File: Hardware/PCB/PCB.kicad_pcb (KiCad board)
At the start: 4 copper layers, 130 x 65 mm, 106 parts, among them IC3 MPX5500DP, IC4 MPX5500DP, J1 DC Motor Terminal, J18 Programmer, J2 Solenoid Terminal, J3 Brushless Vac Motor, J4 54-00127, J5 Brushless Pump Motor, Q1 MMBT2222A, Q2 MMBT2222A, Q3 MMBT2222A, Q4 MMBT2222A, Q5 MMBT2222A, Q6 MMBT2222A, U1 ER-TFTM032-3, U10 AZ1117-5.0, U11 ESP32-S3-WROOM-1U-N16R8, U2 ADS1219IPWR, U3 DRV8871DDA, U4 AP7361C-33E, U5 74LVC2T45DC, U6 TPS7A2050PDBVR, U7 DS3232M, U8 DRV8871DDA

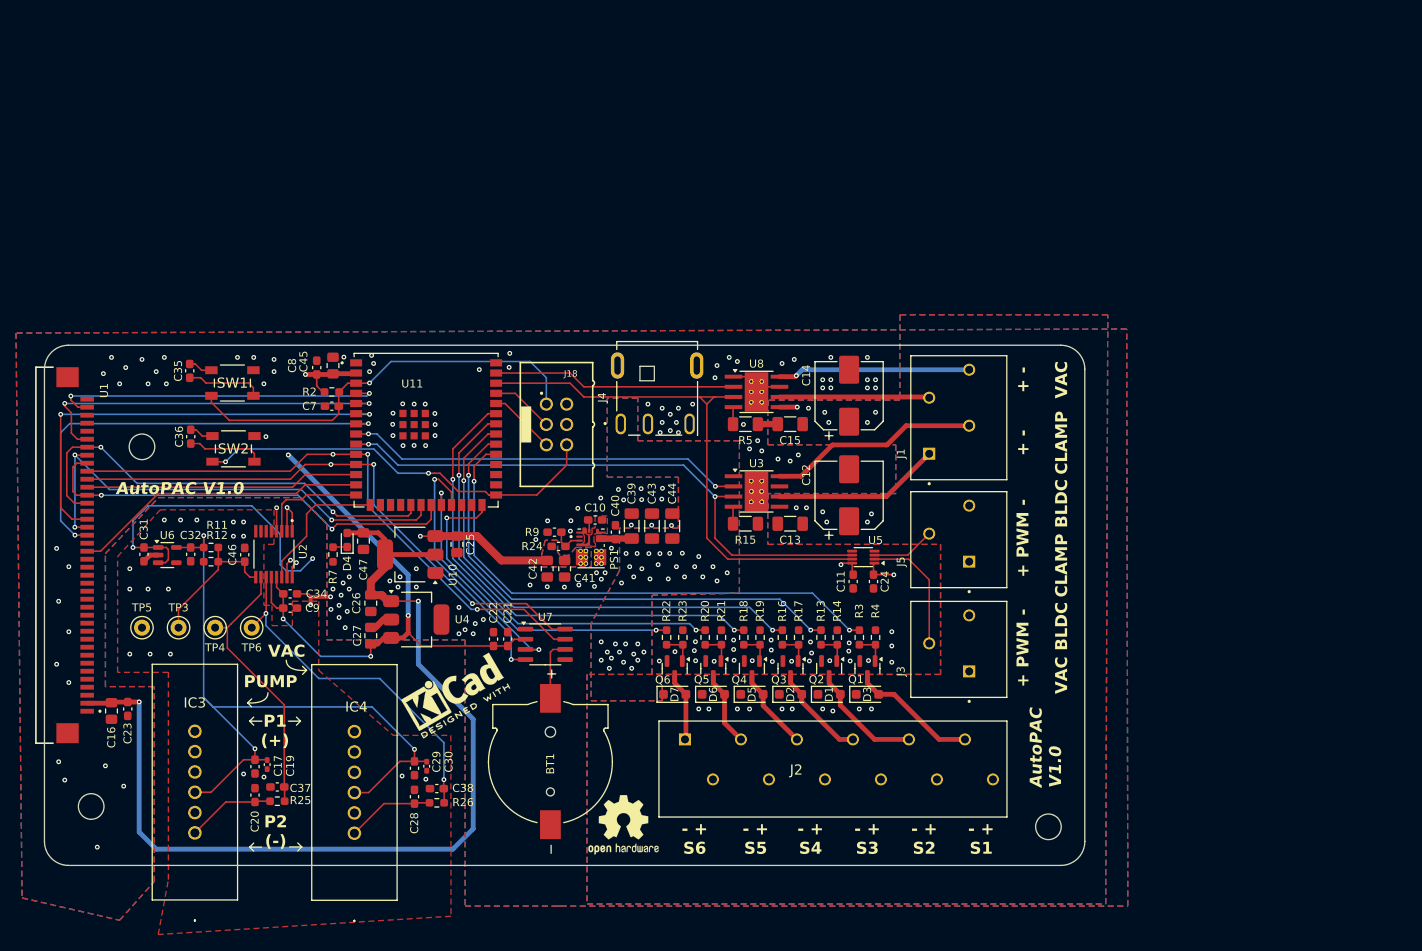
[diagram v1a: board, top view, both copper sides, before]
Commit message: done with this, placed order
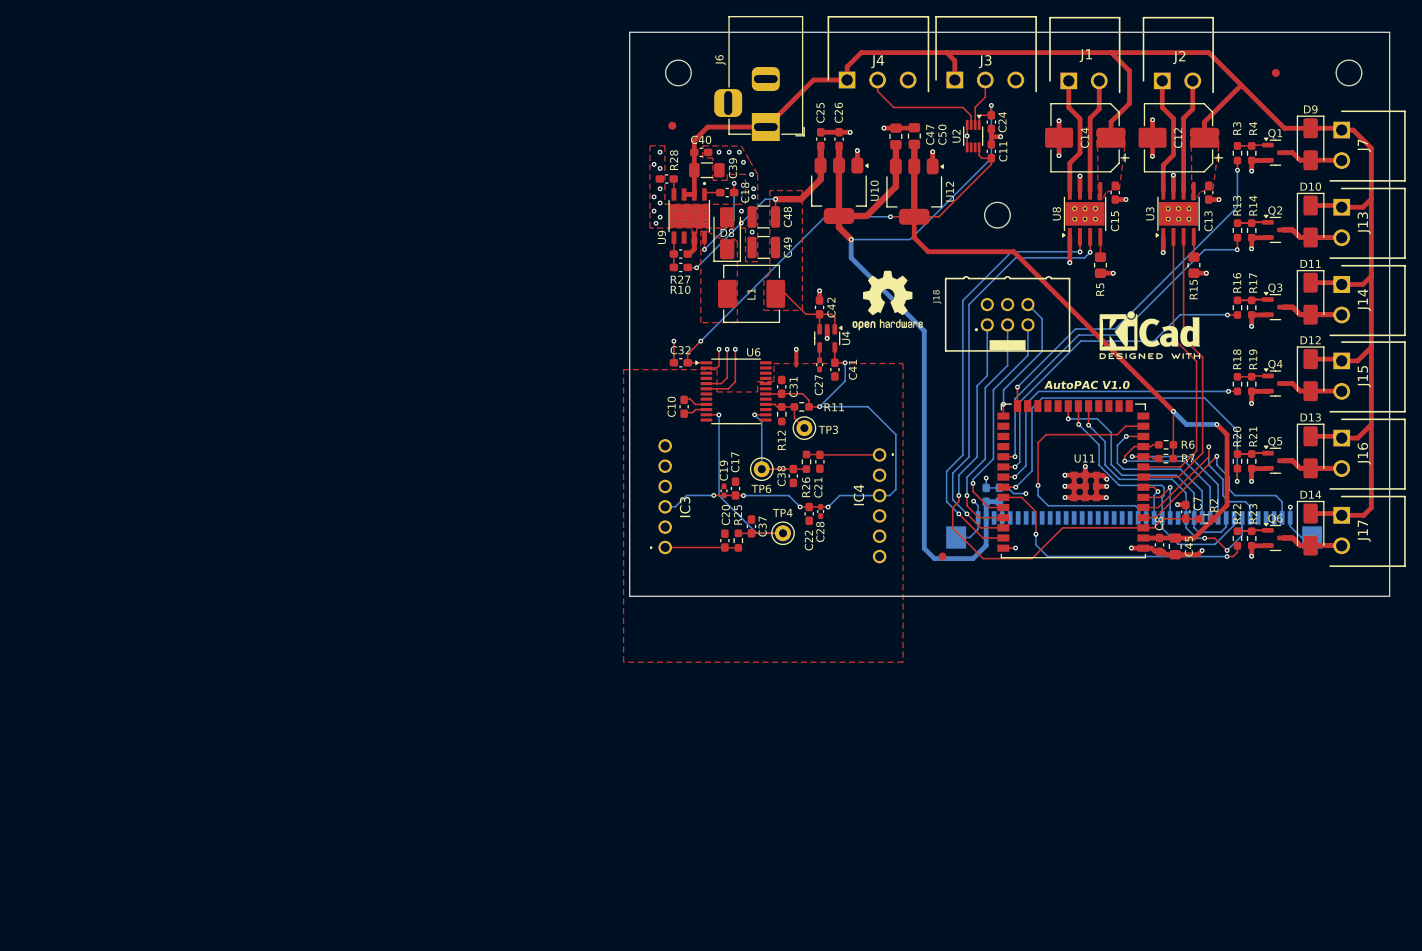
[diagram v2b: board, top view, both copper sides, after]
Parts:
- removed BT1: 1056, Vendor_Footprints:BAT_1056
- removed C29: 1uF, Capacitor_SMD:C_0603_1608Metric_Pad1.08x0.95mm_HandSolder
- removed C30: 0.01uF, Capacitor_SMD:C_0402_1005Metric_Pad0.74x0.62mm_HandSolder
- removed C34, C35, C36, C46, C9: 0.1u, Capacitor_SMD:C_0603_1608Metric_Pad1.08x0.95mm_HandSolder
- removed C43, C44: 10uF, Capacitor_SMD:C_1206_3216Metric_Pad1.33x1.80mm_HandSolder
- removed D1, D2, D3, D5, D6, D7: SMD110PL-TP, Diode_SMD:D_SOD-123F
- removed D4: LED, LED_SMD:LED_0603_1608Metric_Pad1.05x0.95mm_HandSolder
- removed H3: MountingHole, MountingHole:MountingHole_3.2mm_M3
- removed J5: Brushless Pump Motor, Vendor_Footprints:TE_1985205
- removed PS1: TPSM84338RCJR, Vendor_Footprints:CONV_TPSM84338RCJR
- removed R24: 82k, Capacitor_SMD:C_0603_1608Metric_Pad1.08x0.95mm_HandSolder
- removed R9: 10k, Capacitor_SMD:C_0603_1608Metric_Pad1.08x0.95mm_HandSolder
- removed SW1, SW2: ~, Vendor_Footprints:PTS647SN50SMTR2LFS
- removed TP5: TestPoint_Probe, TestPoint:TestPoint_Keystone_5000-5004_Miniature
- removed U5: 74LVC2T45DC, Package_SO:VSSOP-8_2.3x2mm_P0.5mm
- removed U7: DS3232M, Package_SO:SOIC-8_3.9x4.9mm_P1.27mm
- added C18: 100nF, Capacitor_SMD:C_0603_1608Metric_Pad1.08x0.95mm_HandSolder, F.Cu at (187.7, 49.8)
- added C48: 47uF, Capacitor_SMD:C_1210_3225Metric, F.Cu at (192.3, 52.8)
- added C49: 47uF, Capacitor_SMD:C_1210_3225Metric, F.Cu at (192.3, 56.6)
- added C50: 22uF, Capacitor_SMD:C_0805_2012Metric_Pad1.18x1.45mm_HandSolder, F.Cu at (211.1, 42.7)
- added D10: SS310, Diode_SMD:D_SMA, F.Cu at (260.6, 53.4)
- added D11: SS310, Diode_SMD:D_SMA, F.Cu at (260.6, 63.0)
- added D12: SS310, Diode_SMD:D_SMA, F.Cu at (260.6, 72.6)
- added D13: SS310, Diode_SMD:D_SMA, F.Cu at (260.6, 82.2)
- added D14: SS310, Diode_SMD:D_SMA, F.Cu at (260.6, 91.9)
- added D8: SS310, Diode_SMD:D_SMA, F.Cu at (187.7, 54.8)
- added D9: SS310, Diode_SMD:D_SMA, F.Cu at (260.6, 43.7)
- added H2: MountingHole, MountingHole:MountingHole_3.2mm_M3, F.Cu at (221.5, 52.6)
- added J13: Solenoid Terminal, Vendor_Footprints:CONN_WJ15EDGRC-3.81-2P, F.Cu at (264.5, 51.6)
- added J14: Solenoid Terminal, Vendor_Footprints:CONN_WJ15EDGRC-3.81-2P, F.Cu at (264.5, 61.2)
- added J15: Solenoid Terminal, Vendor_Footprints:CONN_WJ15EDGRC-3.81-2P, F.Cu at (264.5, 70.8)
- added J16: Solenoid Terminal, Vendor_Footprints:CONN_WJ15EDGRC-3.81-2P, F.Cu at (264.5, 80.4)
- added J17: Solenoid Terminal, Vendor_Footprints:CONN_WJ15EDGRC-3.81-2P, F.Cu at (264.5, 90.1)
- added J6: XUNPU DC-005-A250, Connector_BarrelJack:BarrelJack_Horizontal, F.Cu at (192.5, 41.6)
- added J7: Solenoid Terminal, Vendor_Footprints:CONN_WJ15EDGRC-3.81-2P, F.Cu at (264.5, 41.9)
- added L1: 6.8uH, Inductor_SMD:L_Changjiang_FXL0630, F.Cu at (190.8, 62.4)
- added R10: 66.5k, Capacitor_SMD:C_0603_1608Metric_Pad1.08x0.95mm_HandSolder, F.Cu at (181.9, 59.1)
- added R27: 10.5k, Capacitor_SMD:C_0603_1608Metric_Pad1.08x0.95mm_HandSolder, F.Cu at (181.9, 57.4)
- added R28: 45.3k, Capacitor_SMD:C_0603_1608Metric_Pad1.08x0.95mm_HandSolder, F.Cu at (180.2, 48.1)
- added R6: 2.2k, Resistor_SMD:R_0603_1608Metric_Pad0.98x0.95mm_HandSolder, F.Cu at (242.6, 81.3)
- added REF**: Fiducial_1mm_Mask3mm, Fiducial:Fiducial_1mm_Mask3mm, F.Cu at (180.8, 41.4)
- added REF**: Fiducial_1mm_Mask3mm, Fiducial:Fiducial_1mm_Mask3mm, F.Cu at (256.3, 34.8)
- added REF**: Fiducial_1mm_Mask3mm, Fiducial:Fiducial_1mm_Mask3mm, F.Cu at (214.6, 95.2)
- added U12: AZ1117-3.3, Package_TO_SOT_SMD:SOT-223-3_TabPin2, F.Cu at (211.1, 49.6)
- added U9: LMR16030PDDAR, Vendor_Footprints:VREG_LM5017MR_NOPB, F.Cu at (183.0, 52.7)
- C10, C11, C24, C8: value 0.1u -> 100nF
- C13, C15: value 0.1uF -> 100nF; footprint Capacitor_SMD:C_1206_3216Metric_Pad1.33x1.80mm_HandSolder -> Capacitor_SMD:C_0603_1608Metric_Pad1.08x0.95mm_HandSolder
- C16: value 10u -> 10uF; footprint Capacitor_SMD:C_0805_2012Metric_Pad1.18x1.45mm_HandSolder -> Capacitor_SMD:C_0603_1608Metric_Pad1.08x0.95mm_HandSolder; moved to B.Cu
- C21: value 1uF -> 470pF
- C22: value 0.1uF -> 1uF
- C23: value 0.1uF -> 100nF; moved to B.Cu
- C25, C26: value 10u -> 10uF; footprint Capacitor_SMD:C_0805_2012Metric_Pad1.18x1.45mm_HandSolder -> Capacitor_SMD:C_0603_1608Metric_Pad1.08x0.95mm_HandSolder
- C27: value 10u -> 0.01uF; footprint Capacitor_SMD:C_0805_2012Metric_Pad1.18x1.45mm_HandSolder -> Capacitor_SMD:C_0402_1005Metric_Pad0.74x0.62mm_HandSolder
- C28: value 470pF -> 0.01uF; footprint Capacitor_SMD:C_0603_1608Metric_Pad1.08x0.95mm_HandSolder -> Capacitor_SMD:C_0402_1005Metric_Pad0.74x0.62mm_HandSolder
- C31, C32: value 1uF -> 100nF
- C40: value 0.1uF -> 100nF
- C41, C42: value 22uF -> 1uF; footprint Capacitor_SMD:C_0805_2012Metric_Pad1.18x1.45mm_HandSolder -> Capacitor_SMD:C_0603_1608Metric_Pad1.08x0.95mm_HandSolder
- C7: value 1u -> 1uF
- J1: value DC Motor Terminal -> Pump Motor; footprint Vendor_Footprints:TE_1985218 -> Vendor_Footprints:CONN_WJ15EDGRC-3.81-2P
- J2: value Solenoid Terminal -> Pump Motor; footprint Vendor_Footprints:PHX_16PIN_1985292 -> Vendor_Footprints:CONN_WJ15EDGRC-3.81-2P
- J3: value Brushless Vac Motor -> BLDC Motor; footprint Vendor_Footprints:TE_1985205 -> Vendor_Footprints:CONN_WJ15EDGRC-3.81-3P
- J4: value 54-00127 -> BLDC Motor; footprint Vendor_Footprints:TENSILITY_54-00127 -> Vendor_Footprints:CONN_WJ15EDGRC-3.81-3P
- R15, R5: footprint Resistor_SMD:R_1206_3216Metric_Pad1.30x1.75mm_HandSolder -> Resistor_SMD:R_0805_2012Metric_Pad1.20x1.40mm_HandSolder
- R7: value 470 -> 2.2k
- U1: moved to B.Cu
- U2: value ADS1219IPWR -> SN74LVC2T45DCUR; footprint Vendor_Footprints:SOP65P640X120-16N -> Package_SO:VSSOP-8_2.3x2mm_P0.5mm
- U4: value AP7361C-33E -> SPX5205M5-L-5-0/TR; footprint Package_TO_SOT_SMD:SOT-223-3_TabPin2 -> Package_TO_SOT_SMD:SOT-23-5
- U6: value TPS7A2050PDBVR -> ADS1232IPW; footprint Package_TO_SOT_SMD:SOT-23-5 -> Package_SO:TSSOP-24_6.1x7.8mm_P0.65mm
- moved H4 157.9 mm to (265.4, 34.8)
- moved U1 133.3 mm to (238.6, 92.9), turned to 180 degrees
- moved H1 117.5 mm to (181.6, 34.8)
- moved C16 114.2 mm to (221.7, 87.5), turned to -90 degrees
- moved C23 110.6 mm to (220.1, 87.5), turned to -90 degrees
- moved R2 110.4 mm to (247.6, 90.6), turned to 180 degrees
- moved C45 107.7 mm to (243.7, 94.0), turned to 90 degrees
- moved C8 107.7 mm to (241.7, 93.8), turned to 90 degrees
- moved C7 107.6 mm to (245.0, 89.7), turned to -90 degrees
- moved R7 104.8 mm to (242.5, 83.0), turned to 180 degrees
- moved U2 101.8 mm to (218.5, 42.7)
- moved J2 101.7 mm to (242.1, 35.8)
- moved REF** 97.7 mm to (240.5, 67.6), turned to 0 degrees
- moved C47 83.6 mm to (208.8, 42.7), turned to 90 degrees
- moved C31 82.4 mm to (194.5, 74.0)
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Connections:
- net /ESP32-S3/GPIO9 renamed /GPIO9
- C10 pad 1: Net-(PS1-SS/PG) -> Net-(C10-Pad1)
- C10 pad 2: GND -> Net-(C10-Pad2)
- C21 pad 1: +3.3V -> GNDA
- C21 pad 2: GND -> Net-(IC4-VOUT)
- C22 pad 1: GND -> +5VA
- C22 pad 2: +3.3V -> GNDA
- C27 pad 1: +3.3V -> GNDA
- C27 pad 2: GND -> Net-(U4-BP)
- C28 pad 1: GNDA -> +5VA
- C28 pad 2: Net-(IC4-VOUT) -> GNDA
- C31 pad 1: GNDA -> +5VA
- C31 pad 2: +5.5V -> GNDA
- C32 pad 1: GNDA -> +3.3V
- C32 pad 2: +5VA -> GND
- C37 pad 2: /sensors/CLAMP_SENSOR -> /sensors/pressure_sensor/SENSOR_VOUT
- C38 pad 2: /sensors/VAC_SENSOR -> /sensors/pressure_sensor1/SENSOR_VOUT
- C41 pad 1: +5.5V -> GNDA
- C41 pad 2: GND -> +5VA
- C42 pad 1: +5.5V -> GND
- C42 pad 2: GND -> +5.5V
- J1 pad 1: /motor_driver1/MOTOR-OUT-1 -> Net-(J1-Pin_1)
- J1 pad 2: /motor_driver1/MOTOR-OUT-2 -> Net-(J1-Pin_2)
- J2 pad 1: /relay_driver5/COIL- -> Net-(J2-Pin_1)
- J2 pad 2: +24V -> Net-(J2-Pin_2)
- J3 pad 2: /brushless_motor_pwm_driver/BRUSHLESS_PWM_1 -> Net-(J3-Pin_2)
- Q1 pad 3: /relay_driver/COIL- -> Net-(D9-A)
- Q2 pad 3: /relay_driver1/COIL- -> Net-(D10-A)
- Q3 pad 3: /relay_driver2/COIL- -> Net-(D11-A)
- Q4 pad 3: /relay_driver3/COIL- -> Net-(D12-A)
- Q5 pad 3: /relay_driver4/COIL- -> Net-(D13-A)
- Q6 pad 3: /relay_driver5/COIL- -> Net-(D14-A)
- R25 pad 2: /sensors/CLAMP_SENSOR -> /sensors/pressure_sensor/SENSOR_VOUT
- R26 pad 2: /sensors/VAC_SENSOR -> /sensors/pressure_sensor1/SENSOR_VOUT
- R7 pad 1: Net-(D4-K) -> +3.3V
- R7 pad 2: GND -> /I2C-SDA
- TP4 pad 1: /sensors/CLAMP_SENSOR -> /sensors/pressure_sensor/SENSOR_VOUT
- TP6 pad 1: /sensors/VAC_SENSOR -> /sensors/pressure_sensor1/SENSOR_VOUT
- U11 pad 14: /ADC-RESET -> /GPIO20
- U11 pad 15: /ADC-DRDY -> /GPIO3
- U11 pad 22: /RTC-INT -> /GPIO14
- U11 pad 23: /RTC-RESET -> /GPIO21
- U11 pad 26: /SOLENOID_6 -> /SOLENOID_1
- U11 pad 31: /SOLENOID_1 -> /SOLENOID_2
- U11 pad 32: /SOLENOID_2 -> /SOLENOID_3
- U11 pad 33: /SOLENOID_3 -> /SOLENOID_4
- U11 pad 34: /SOLENOID_4 -> /SOLENOID_5
- U11 pad 35: /SOLENOID_5 -> /SOLENOID_6
- U11 pad 8: /PUMP-IN2 -> /PUMP-IN1
- U11 pad 9: /PUMP-IN1 -> /PUMP-IN2
- U2 pad 1: GND -> +5V
- U2 pad 2: GND -> Net-(J3-Pin_2)
- U2 pad 3: /ADC-RESET -> Net-(J4-Pin_2)
- U2 pad 5: GNDA -> GND
- U2 pad 6: unconnected-(U2-AIN3-Pad6) -> /brushless_motor_pwm_driver/Pump_PWM
- U2 pad 7: unconnected-(U2-AIN2-Pad7) -> /brushless_motor_pwm_driver/Vac_PWM
- U2 pad 8: GNDA -> +3.3V
- U3 pad 6: /motor_driver1/MOTOR-OUT-1 -> Net-(J2-Pin_2)
- U3 pad 8: /motor_driver1/MOTOR-OUT-2 -> Net-(J2-Pin_1)
- U4 pad 1: +5V -> +5.5V
- U4 pad 3: +3.3V -> +5.5V
- U6 pad 1: +5.5V -> +3.3V
- U6 pad 2: GNDA -> GND
- U6 pad 3: +5.5V -> GNDA
- U6 pad 5: +5VA -> GND
- U8 pad 6: /motor_driver/MOTOR-OUT-1 -> Net-(J1-Pin_2)
- U8 pad 8: /motor_driver/MOTOR-OUT-2 -> Net-(J1-Pin_1)
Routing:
- net +24V: track 6.40 -> 217.1 mm, vias 57 -> 0
- net GND: track 27.4 -> 142.6 mm, vias 151 -> 64
- net /I2C-SDA: track 91.8 -> 19.8 mm, vias 4 -> 1
- net +5V: track 188.0 -> 116.9 mm, vias 3 -> 2
- net /I2C-SCL: track 88.1 -> 21.4 mm, vias 4 -> 1
- net /DISP-CS: track 55.6 -> 5.57 mm, vias 2 -> 1
- net /DISP-DC: track 55.9 -> 7.68 mm, vias 2 -> 1
- net /sensors/VAC_SENSOR: track 44.4 -> 0.00 mm, vias 2 -> 0
- net /PUMP-IN1: track 73.1 -> 36.7 mm, vias 2 -> 0
- net /ESP32-S3/BOOT: track 51.4 -> 16.7 mm, vias 2 -> 1
- net /sensors/CLAMP_SENSOR: track 34.2 -> 0.00 mm
- net /RTC-RESET: track 32.7 -> 0.00 mm, vias 2 -> 0
- net +5.5V: track 71.8 -> 39.6 mm
- net /RTC-INT: track 28.3 -> 0.00 mm, vias 2 -> 0
- net /sensors/pressure_sensor/SENSOR_VOUT: track 0.00 -> 27.2 mm, vias 0 -> 1
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- added copper zone on F.Cu, net Net-(D8-K)
- removed copper zone on B.Cu, net +24V
- removed copper zone on B.Cu, net +5.5V
- removed copper zone on B.Cu, net GND
- removed copper zone on In1.Cu, net GNDA
- removed copper zone on In2.Cu, net GNDA
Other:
- board size 130 x 65 mm -> 95 x 70.5 mm
- board text removed: "+ - CLAMP"
- board text removed: "+ - VAC"
- board text removed: "+ PWM - CLAMP BLDC"
- board text removed: "+ PWM - VAC BLDC"
- board text removed: "- + S1"
- board text removed: "- + S2"
- board text removed: "- + S3"
- board text removed: "- + S4"
- board text removed: "- + S5"
- board text removed: "- + S6"
- board text removed: "P1 (+)"
- board text removed: "P2 (-)"
- board text removed: "PUMP"
- board text removed: "VAC"
